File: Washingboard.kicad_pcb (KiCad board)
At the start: 2 copper layers, 3 parts, among them U1 RT9080-33GJ5, U2 ESP32-S3-MINI-1

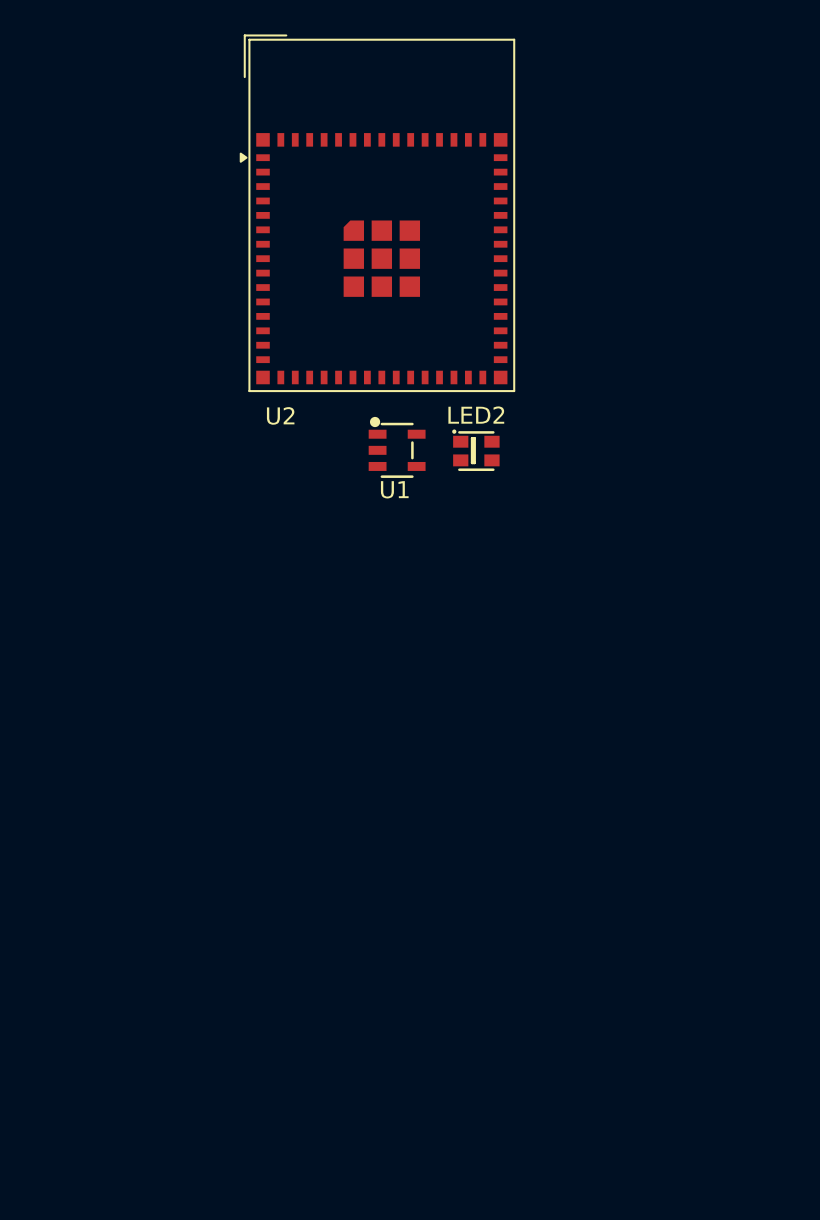
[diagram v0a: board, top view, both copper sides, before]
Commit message: PCB Layout
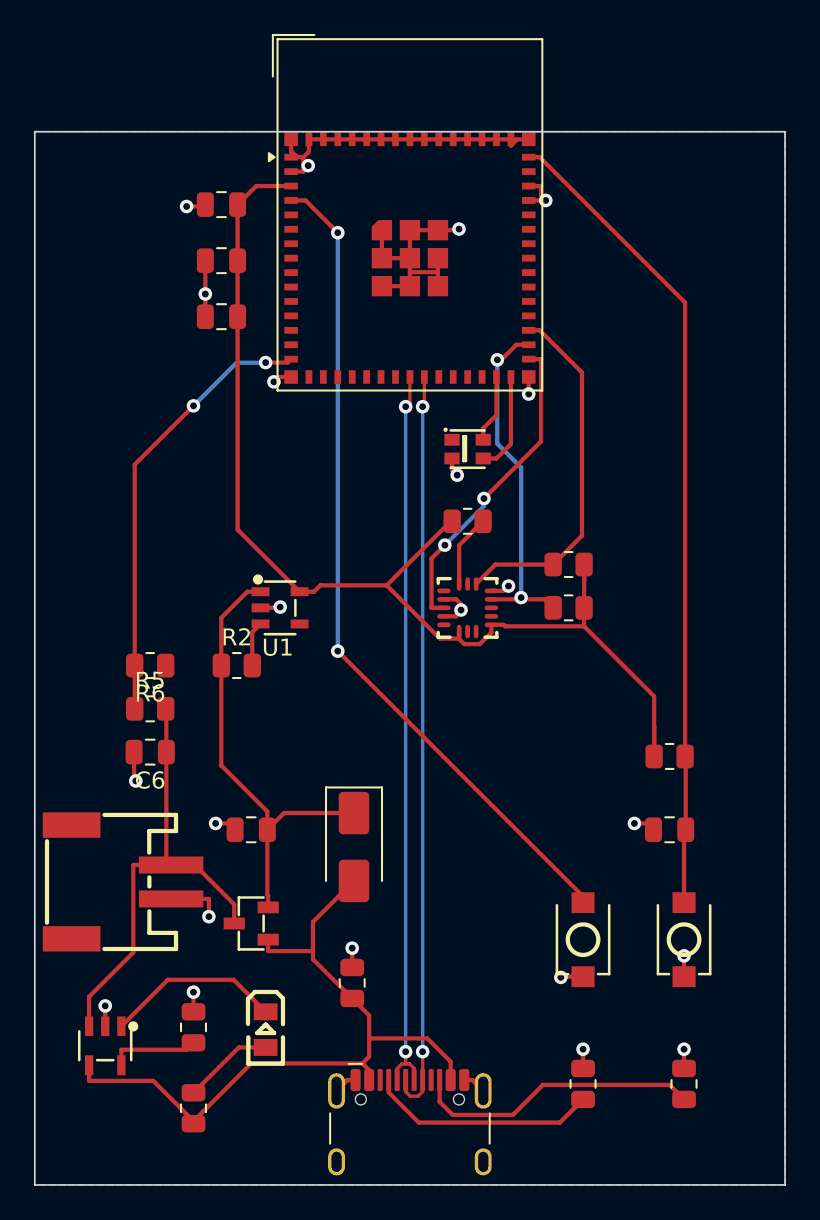
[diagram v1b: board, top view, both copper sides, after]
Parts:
- added C1: 10uF, Capacitor_SMD:C_0805_2012Metric, F.Cu at (118.2, 90.4)
- added C2: 10uF, Capacitor_SMD:C_0805_2012Metric, F.Cu at (116.4, 60.2)
- added C3: 10uF, Capacitor_SMD:C_0805_2012Metric, F.Cu at (116.4, 56.9)
- added C4: 0.1uF, Capacitor_SMD:C_0805_2012Metric, F.Cu at (116.4, 53.6)
- added C5: 10uF, Capacitor_SMD:C_0805_2012Metric, F.Cu at (142.8, 90.4)
- added C6: 10uF, Capacitor_SMD:C_0805_2012Metric, F.Cu at (112.2, 85.8)
- added CN1: JST S2B-PH-SM4-TB(LF)(SN), easyeda2kicad:CONN-SMD_P2.00_S2B-PH-SM4-TB-LF-SN, F.Cu at (110.5, 93.5)
- added D1: SK54A-LTP, Diode_SMD:D_SMA, F.Cu at (124.2, 91.4)
- added J2: HCTL HC-TYPE-C-16P-01A, Connector_USB:USB_C_Receptacle_HCTL_HC-TYPE-C-16P-01A, F.Cu at (127.5, 108.9)
- added LED1: FC-2012HRK-620D, easyeda2kicad:LED0805-R-RD, F.Cu at (119.0, 102.2)
- added Q1: DMP2045UQ-7, easyeda2kicad:SOT-23-3_L2.9-W1.3-P0.95-LS2.4-BR, F.Cu at (118.2, 95.9)
- added R1: 100K, Resistor_SMD:R_0805_2012Metric, F.Cu at (124.1, 99.5)
- added R10: 5.1K, Resistor_SMD:R_0805_2012Metric, F.Cu at (136.8, 77.3)
- added R11: 160, Resistor_SMD:R_0805_2012Metric, F.Cu at (114.8, 106.8)
- added R12: 2k, Resistor_SMD:R_0805_2012Metric, F.Cu at (114.8, 102.1)
- added R2: 100K, Resistor_SMD:R_0805_2012Metric, F.Cu at (117.3, 80.8)
- added R3: 5.1K, Resistor_SMD:R_0805_2012Metric, F.Cu at (143.7, 105.4)
- added R4: 5.1K, Resistor_SMD:R_0805_2012Metric, F.Cu at (137.7, 105.4)
- added R5: 470K, Resistor_SMD:R_0805_2012Metric, F.Cu at (112.2, 83.3)
- added R6: 470K, Resistor_SMD:R_0805_2012Metric, F.Cu at (112.2, 80.8)
- added R7: 5.1K, Resistor_SMD:R_0805_2012Metric, F.Cu at (142.8, 86.1)
- added R8: 5.1K, Resistor_SMD:R_0805_2012Metric, F.Cu at (130.9, 72.2)
- added R9: 5.1K, Resistor_SMD:R_0805_2012Metric, F.Cu at (136.8, 74.8)
- added SW1: TS-1088-AR02016, easyeda2kicad:SW-SMD_L3.9-W3.0-P4.45, F.Cu at (143.7, 96.9)
- added SW2: TS-1088-AR02016, easyeda2kicad:SW-SMD_L3.9-W3.0-P4.45, F.Cu at (137.7, 96.9)
- added U3: LIS3DHTR_C15134, easyeda2kicad:LGA-16_L3.0-W3.0-P0.50-TL, F.Cu at (130.9, 77.3)
- added U4: MCP73831T-2ACI/OT, easyeda2kicad:SOT-23-5_L3.0-W1.7-P0.95-LS2.8-BL, F.Cu at (109.5, 103.2)
- moved U1 11.6 mm to (119.8, 77.3)
- moved U2 1.66 mm to (127.5, 54.2)
- moved LED2 0.53 mm to (130.9, 68.0)
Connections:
- LED2 pad 2: unconnected-(LED2-GND-Pad2) -> GND
- LED2 pad 3: unconnected-(LED2-DI-Pad3) -> NEOPIXEL
- LED2 pad 4: unconnected-(LED2-VDD-Pad4) -> NEOPIXELPWR
- U1 pad 1: unconnected-(U1-VIN-Pad1) -> Net-(D1-K)
- U1 pad 2: unconnected-(U1-GND-Pad2) -> GND
- U1 pad 3: unconnected-(U1-EN-Pad3) -> Net-(U1-EN)
- U1 pad 5: unconnected-(U1-VOUT-Pad5) -> 3.3V
- U2 pad 1: Net-(U2-GND-Pad1) -> GND
- U2 pad 15: unconnected-(U2-IO11-Pad15) -> GPIO1
- U2 pad 2: Net-(U2-GND-Pad1) -> GND
- U2 pad 23: unconnected-(U2-IO19-Pad23) -> D-
- U2 pad 24: unconnected-(U2-IO20-Pad24) -> D+
- U2 pad 29: unconnected-(U2-IO34-Pad29) -> NEOPIXELPWR
- U2 pad 3: unconnected-(U2-3V3-Pad3) -> 3.3V
- U2 pad 30: unconnected-(U2-IO48-Pad30) -> NEOPIXEL
- U2 pad 31: unconnected-(U2-IO35-Pad31) -> INT1
- U2 pad 32: unconnected-(U2-IO36-Pad32) -> SCL
- U2 pad 33: unconnected-(U2-IO37-Pad33) -> SDA
- U2 pad 4: unconnected-(U2-IO0-Pad4) -> BOOT
- U2 pad 42: Net-(U2-GND-Pad1) -> GND
- U2 pad 43: Net-(U2-GND-Pad1) -> GND
- U2 pad 45: unconnected-(U2-EN-Pad45) -> RESET
- U2 pad 46: Net-(U2-GND-Pad1) -> GND
- U2 pad 47: Net-(U2-GND-Pad1) -> GND
- U2 pad 48: Net-(U2-GND-Pad1) -> GND
- U2 pad 49: Net-(U2-GND-Pad1) -> GND
- U2 pad 50: Net-(U2-GND-Pad1) -> GND
- U2 pad 51: Net-(U2-GND-Pad1) -> GND
- U2 pad 52: Net-(U2-GND-Pad1) -> GND
- U2 pad 53: Net-(U2-GND-Pad1) -> GND
- U2 pad 54: Net-(U2-GND-Pad1) -> GND
- U2 pad 55: Net-(U2-GND-Pad1) -> GND
- U2 pad 56: Net-(U2-GND-Pad1) -> GND
- U2 pad 57: Net-(U2-GND-Pad1) -> GND
- U2 pad 58: Net-(U2-GND-Pad1) -> GND
- U2 pad 59: Net-(U2-GND-Pad1) -> GND
- U2 pad 60: Net-(U2-GND-Pad1) -> GND
- U2 pad 61: Net-(U2-GND-Pad1) -> GND
- U2 pad 62: Net-(U2-GND-Pad1) -> GND
- U2 pad 63: Net-(U2-GND-Pad1) -> GND
- U2 pad 64: Net-(U2-GND-Pad1) -> GND
- U2 pad 65: Net-(U2-GND-Pad1) -> GND
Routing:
- net 3.3V: track 0.00 -> 67.6 mm
- net GND: track 0.00 -> 64.8 mm, vias 0 -> 22
- net BOOT: track 0.00 -> 48.6 mm, vias 0 -> 2
- net RESET: track 0.00 -> 48.0 mm
- net D+: track 0.00 -> 44.0 mm, vias 0 -> 2
- net VBUS: track 0.00 -> 43.6 mm
- net D-: track 0.00 -> 43.2 mm, vias 0 -> 2
- net Net-(D1-K): track 0.00 -> 26.7 mm
- net GPIO1: track 0.00 -> 26.2 mm, vias 0 -> 2
- net VBAT: track 0.00 -> 26.1 mm
- net SDA: track 0.00 -> 21.2 mm
- net SCL: track 0.00 -> 20.8 mm, vias 0 -> 2
- net INT1: track 0.00 -> 18.8 mm, vias 0 -> 2
- net Net-(J2-CC2): track 0.00 -> 17.7 mm
- net Net-(J2-CC1): track 0.00 -> 14.4 mm
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- added copper zone on B.Cu, net GND
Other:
- board outline added: 44.2 x 62 mm
